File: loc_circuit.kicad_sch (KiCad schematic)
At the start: 4 parts, among them U1 ATmega2560-16A, Y1 16MHz

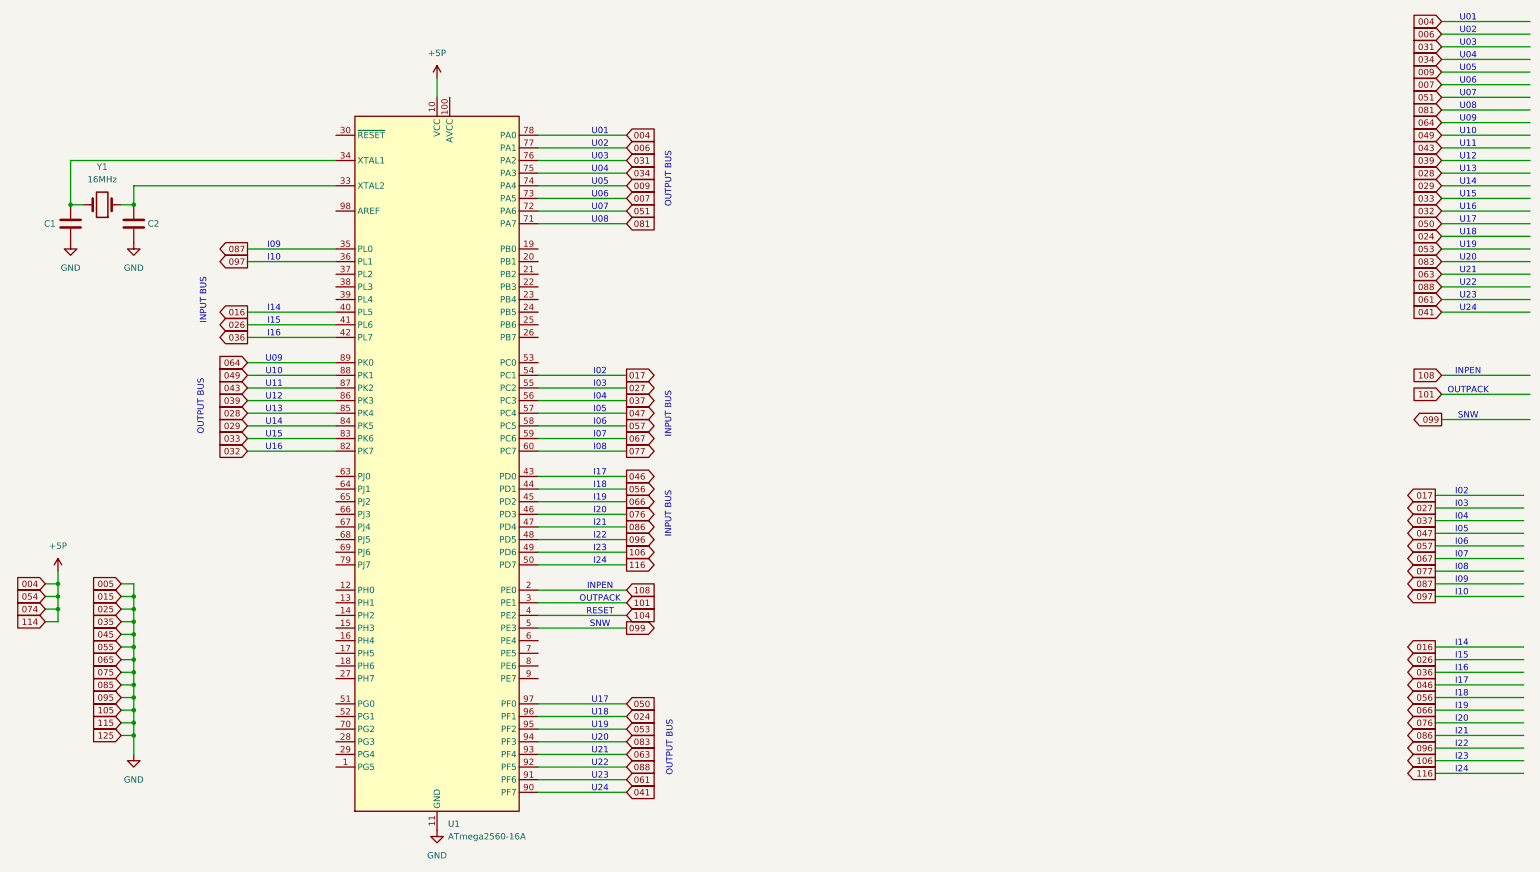
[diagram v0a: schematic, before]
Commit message: Add files via upload
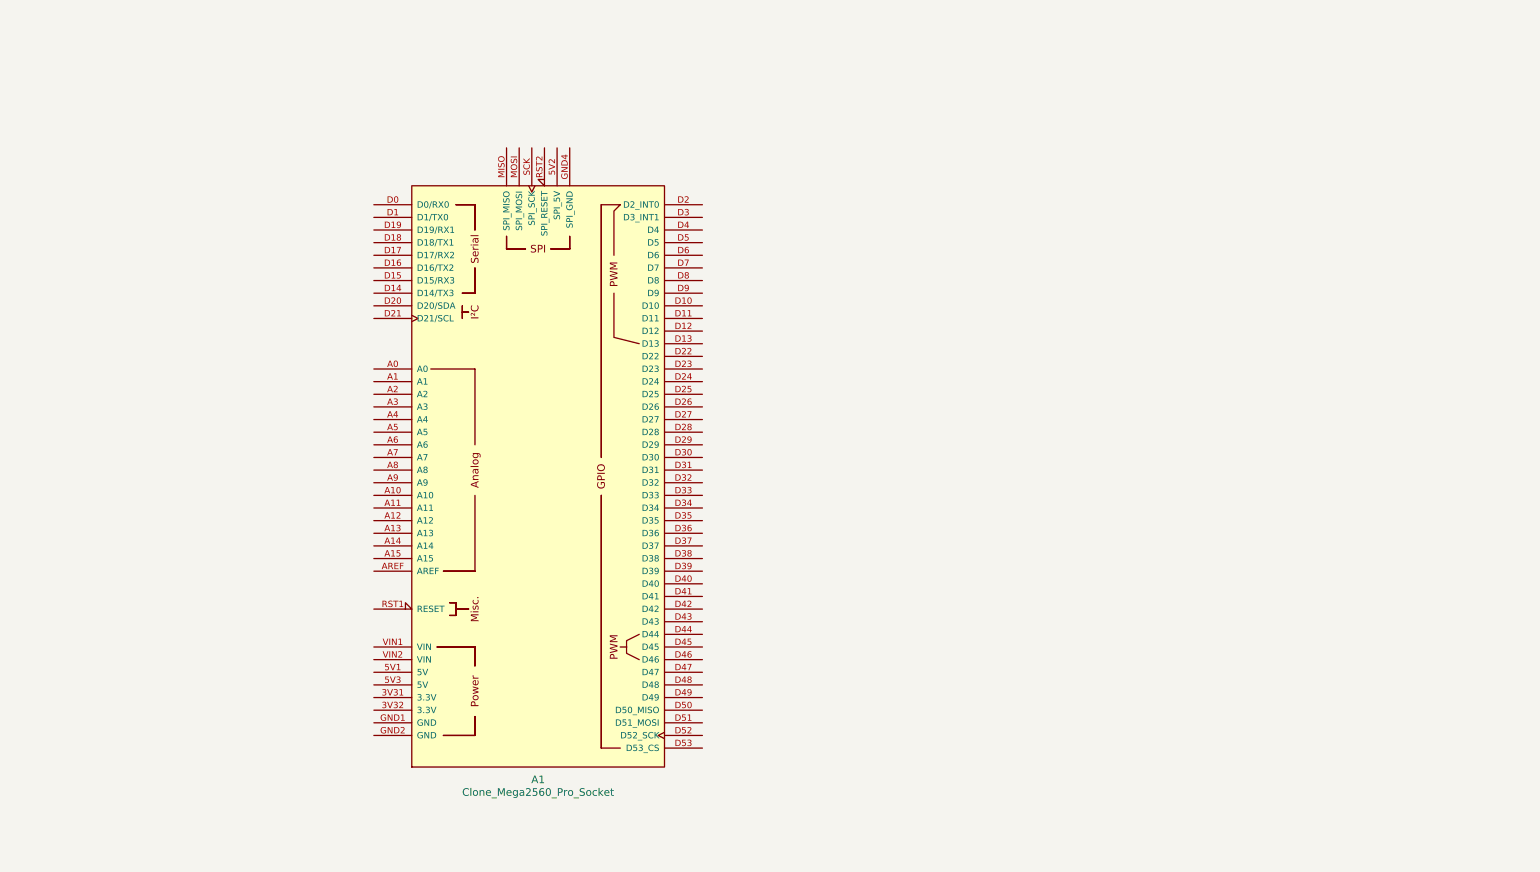
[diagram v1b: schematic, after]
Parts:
- removed C1, C2: C, symbol Device:C
- removed U1: ATmega2560-16A, Package_QFP:TQFP-100_14x14mm_P0.5mm, symbol MCU_Microchip_ATmega:ATmega2560-16A
- removed Y1: 16MHz, symbol Device:Crystal
- added A1: Clone_Mega2560_Pro_Socket, PCM_arduino-library:Clone_Mega2560_Pro_Socket, symbol arduino-library:Clone_Mega2560_Pro_Socket
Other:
- note removed: "I02"
- note removed: "I03"
- note removed: "I04"
- note removed: "I05"
- note removed: "I06"
- note removed: "I07"
- note removed: "I08"
- note removed: "I09"
- note removed: "I10"
- note removed: "I14"
- note removed: "I15"
- note removed: "I16"
- note removed: "I17"
- note removed: "I18"
- note removed: "I19"
- note removed: "I20"
- note removed: "I21"
- note removed: "I22"
- note removed: "I23"
- note removed: "I24"
- note removed: "INPEN"
- note removed: "INPUT BUS"
- note removed: "OUTPACK"
- note removed: "OUTPUT BUS"
- note removed: "RESET"
- note removed: "SNW"
- note removed: "U01"
- note removed: "U02"
- note removed: "U03"
- note removed: "U04"
- note removed: "U05"
- note removed: "U06"
- note removed: "U07"
- note removed: "U08"
- note removed: "U09"
- note removed: "U10"
- note removed: "U11"
- note removed: "U12"
- note removed: "U13"
- note removed: "U14"
- note removed: "U15"
- note removed: "U16"
- note removed: "U17"
- note removed: "U18"
- note removed: "U19"
- note removed: "U20"
- note removed: "U21"
- note removed: "U22"
- note removed: "U23"
- note removed: "U24"
